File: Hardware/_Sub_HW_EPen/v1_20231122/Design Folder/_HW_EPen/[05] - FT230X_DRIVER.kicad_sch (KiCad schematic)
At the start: 13 parts, among them U501 FT230XQ-R

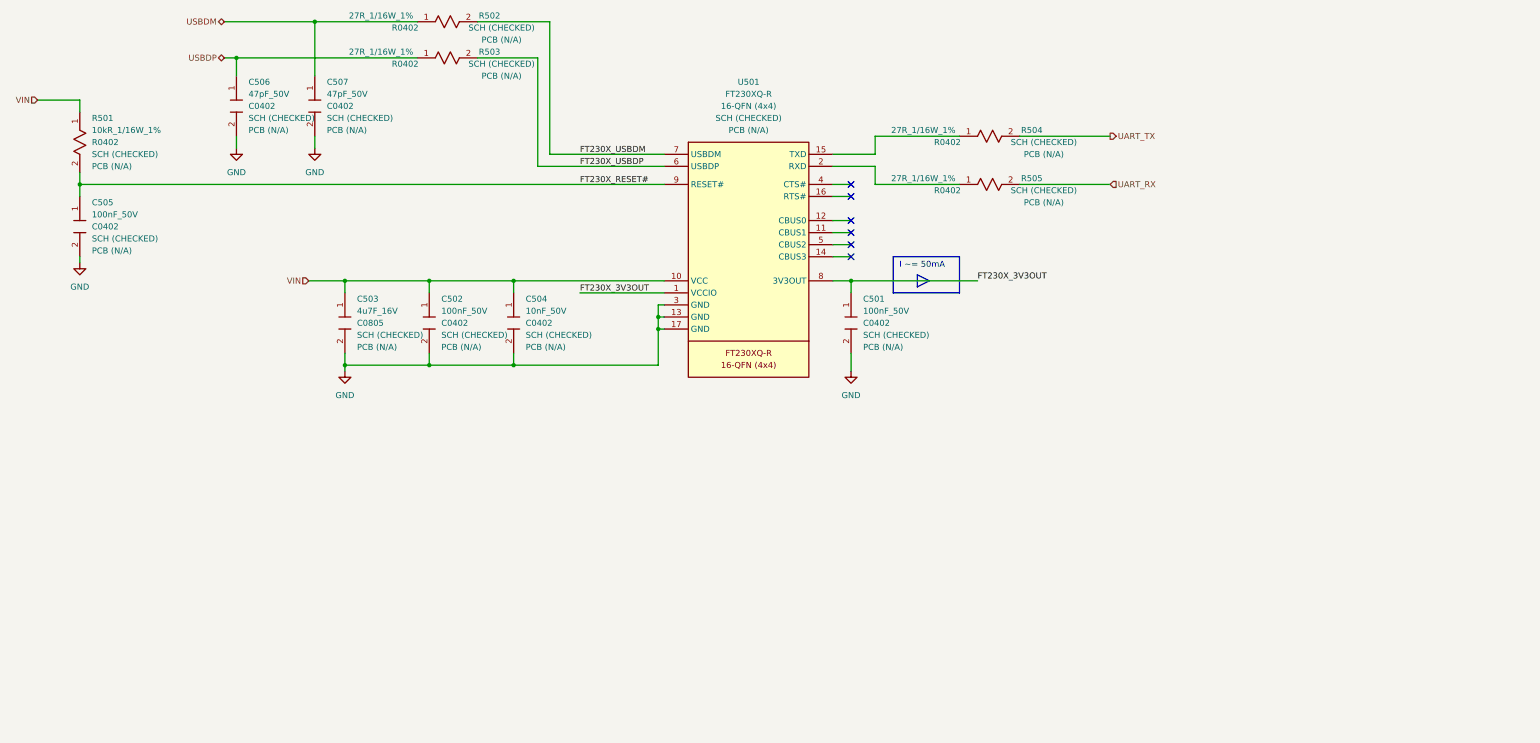
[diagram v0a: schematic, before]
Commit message: Updating file templates and structures...
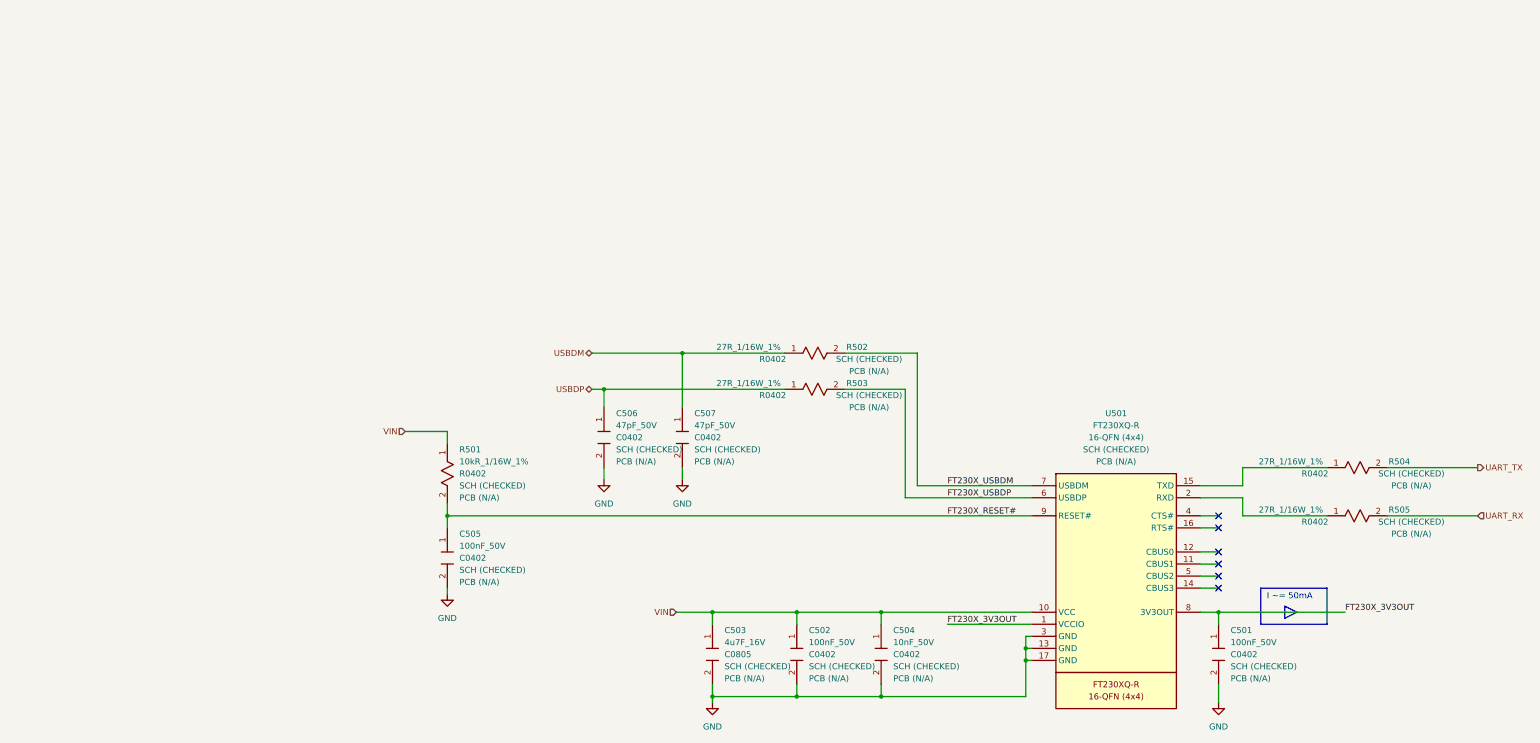
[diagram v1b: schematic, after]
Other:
- moved on the sheet: C501, C502, C503, C504, C505, C506, C507, R501, R502, R503, R504, R505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

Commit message: Updating Hardware File structures
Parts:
- C501, C502, C505: Manufacturer (none) -> Murata Electronics; Part Number GRM155R71H104KE14J -> (none); Part Number (Manufacturer) (none) -> GRM155R71H104KE14J; Part Number (Vendor) (none) -> 490-13342-2-ND; Vendor (none) -> Digikey
- C503: Manufacturer (none) -> Murata Electronics; Part Number GRM21BR71C475KE51L -> (none); Part Number (Manufacturer) (none) -> GRM21BR71C475KE51L; Part Number (Vendor) (none) -> 490-14466-2-ND; Vendor (none) -> Digikey
- C504: Manufacturer (none) -> Samsung Electro-Mechanics; Part Number CL05B103KB5NNNC -> (none); Part Number (Manufacturer) (none) -> CL05B103KB5NNNC; Part Number (Vendor) (none) -> 1276-1028-2-ND; Vendor (none) -> Digikey
- C506, C507: Manufacturer (none) -> KEMET; Part Number C0402C470J5RACAUTO -> (none); Part Number (Manufacturer) (none) -> C0402C470J5RACAUTO; Part Number (Vendor) (none) -> 399-C0402C470J5RACAUTOTR-ND; Vendor (none) -> Digikey
- R501: Manufacturer (none) -> Bourns Inc.; Part Number CR0402-FX-1002GLF -> (none); Part Number (Manufacturer) (none) -> CR0402-FX-1002GLF; Part Number (Vendor) (none) -> CR0402-FX-1002GLFTR-ND; Vendor (none) -> Digikey
- R502, R503, R504, R505: Manufacturer (none) -> Bourns Inc.; Part Number CR0402-FX-27R0GLF -> (none); Part Number (Manufacturer) (none) -> CR0402-FX-27R0GLF; Part Number (Vendor) (none) -> CR0402-FX-27R0GLFTR-ND; Vendor (none) -> Digikey
- U501: Manufacturer (none) -> FTDI, Future Technology Devices International Ltd; Part Number FT230XQ-R -> (none); Part Number (Manufacturer) (none) -> FT230XQ-R; Part Number (Vendor) (none) -> 768-1130-2-ND; Vendor (none) -> Digikey
